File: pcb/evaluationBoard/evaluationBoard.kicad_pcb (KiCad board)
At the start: 2 copper layers, 36 parts, among them IC1 STM32F429ZGT6, IC2 TPS5430DDAR, IC3 TPS54331DR

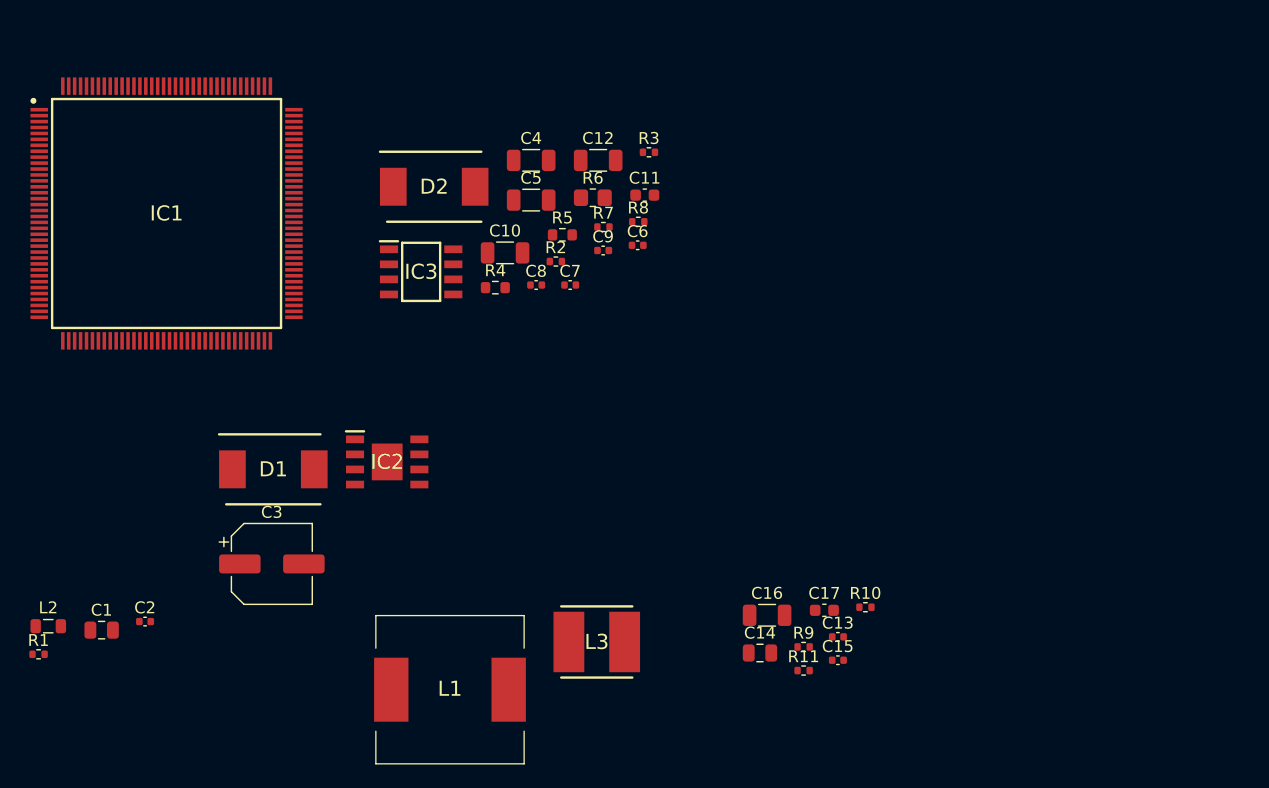
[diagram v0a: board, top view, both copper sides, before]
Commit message: wip
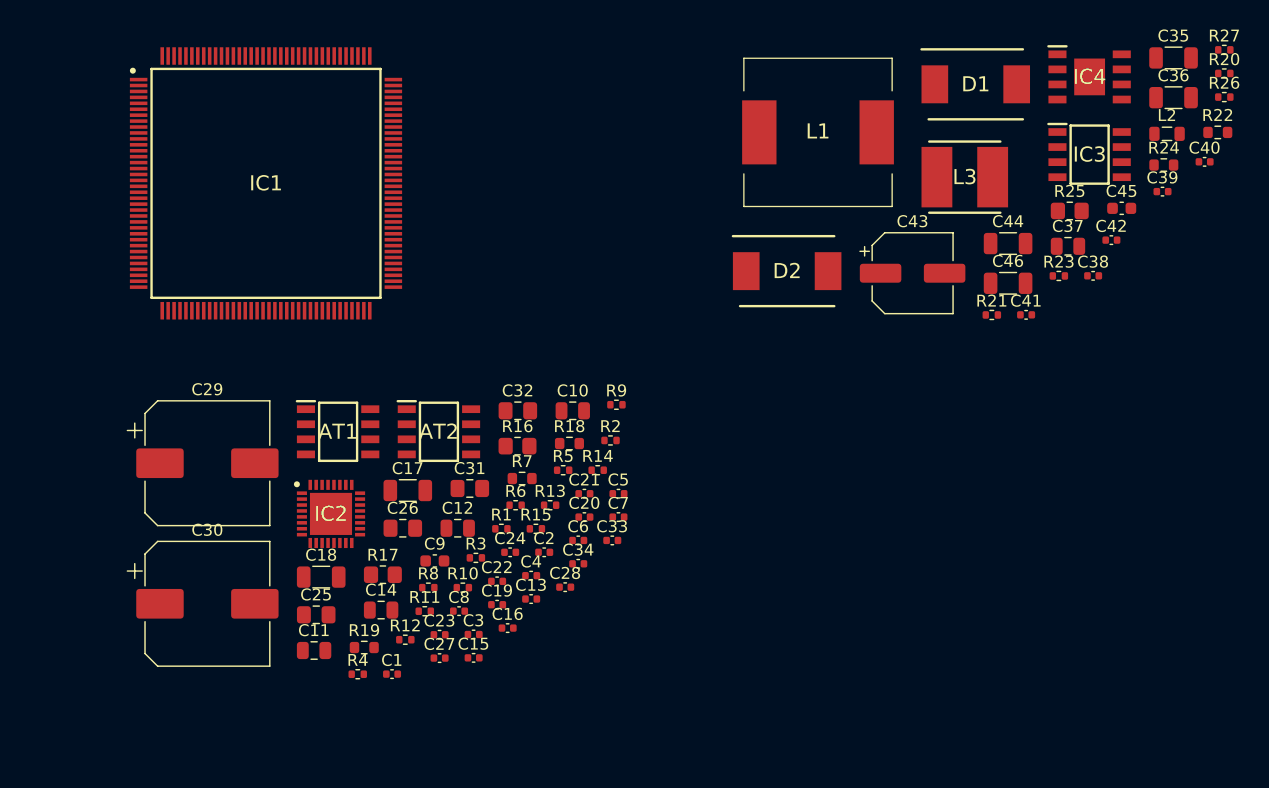
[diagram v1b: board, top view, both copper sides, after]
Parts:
- added AT1: LM386MX-1_NOPB, SOIC127P600X175-8N, F.Cu at (168.2, 72.8)
- added AT2: LM386MX-1_NOPB, SOIC127P600X175-8N, F.Cu at (176.7, 72.8)
- added C18: 47uF, Capacitor_SMD:C_1206_3216Metric, F.Cu at (166.8, 85.1)
- added C19: 4.7n, Capacitor_SMD:C_0402_1005Metric, F.Cu at (181.6, 87.4)
- added C20: 4.7n, Capacitor_SMD:C_0402_1005Metric, F.Cu at (189.0, 80.0)
- added C21: 100n, Capacitor_SMD:C_0402_1005Metric, F.Cu at (189.0, 78.0)
- added C22: 100n, Capacitor_SMD:C_0402_1005Metric, F.Cu at (181.6, 85.4)
- added C23: 100n, Capacitor_SMD:C_0402_1005Metric, F.Cu at (176.8, 89.9)
- added C24: 100n, Capacitor_SMD:C_0402_1005Metric, F.Cu at (182.7, 83.0)
- added C25: NA_C, Capacitor_SMD:C_0805_2012Metric_Pad1.18x1.45mm_HandSolder, F.Cu at (166.4, 88.3)
- added C26: NA_C, Capacitor_SMD:C_0805_2012Metric_Pad1.18x1.45mm_HandSolder, F.Cu at (173.7, 81.0)
- added C27: 47n, Capacitor_SMD:C_0402_1005Metric, F.Cu at (176.8, 91.9)
- added C28: 47n, Capacitor_SMD:C_0402_1005Metric, F.Cu at (187.3, 85.9)
- added C29: 220uF_E, Capacitor_SMD:CP_Elec_10x10, F.Cu at (157.2, 75.5)
- added C30: 220uF_E, Capacitor_SMD:CP_Elec_10x10, F.Cu at (157.2, 87.3)
- added C31: NA_C, Capacitor_SMD:C_0805_2012Metric_Pad1.18x1.45mm_HandSolder, F.Cu at (179.3, 77.6)
- added C32: NA_C, Capacitor_SMD:C_0805_2012Metric_Pad1.18x1.45mm_HandSolder, F.Cu at (183.4, 71.1)
- added C33: 100n, Capacitor_SMD:C_0402_1005Metric, F.Cu at (191.3, 82.0)
- added C34: 100n, Capacitor_SMD:C_0402_1005Metric, F.Cu at (188.4, 84.0)
- added C35: 4.7u, Capacitor_SMD:C_1206_3216Metric, F.Cu at (238.6, 41.3)
- added C36: 4.7u, Capacitor_SMD:C_1206_3216Metric, F.Cu at (238.6, 44.7)
- added C37: 10u, Capacitor_SMD:C_0805_2012Metric, F.Cu at (229.7, 57.2)
- added C38: 10n, Capacitor_SMD:C_0402_1005Metric, F.Cu at (231.9, 59.7)
- added C39: 100n, Capacitor_SMD:C_0402_1005Metric, F.Cu at (237.7, 52.6)
- added C40: 10n, Capacitor_SMD:C_0402_1005Metric, F.Cu at (241.3, 50.1)
- added C41: 10n, Capacitor_SMD:C_0402_1005Metric, F.Cu at (226.2, 63.0)
- added C42: 1n, Capacitor_SMD:C_0402_1005Metric, F.Cu at (233.4, 56.7)
- added C43: 220uF_E, Capacitor_SMD:CP_Elec_6.3x7.7, F.Cu at (216.6, 59.5)
- added C44: 47uF, Capacitor_SMD:C_1206_3216Metric, F.Cu at (224.7, 57.0)
- added C45: 47pF, Capacitor_SMD:C_0603_1608Metric, F.Cu at (234.3, 54.0)
- added C46: 47uF, Capacitor_SMD:C_1206_3216Metric, F.Cu at (224.7, 60.3)
- added IC4: TPS5430DDAR, SOIC127P600X170-9N, F.Cu at (231.6, 42.9)
- added R12: 1k, Resistor_SMD:R_0402_1005Metric, F.Cu at (173.9, 90.4)
- added R13: 2.7k, Resistor_SMD:R_0402_1005Metric, F.Cu at (186.1, 79.0)
- added R14: 1k, Resistor_SMD:R_0402_1005Metric, F.Cu at (190.1, 76.1)
- added R15: 1k, Resistor_SMD:R_0402_1005Metric, F.Cu at (184.9, 81.0)
- added R16: NA_R, Resistor_SMD:R_0805_2012Metric_Pad1.20x1.40mm_HandSolder, F.Cu at (183.3, 74.0)
- added R17: NA_R, Resistor_SMD:R_0805_2012Metric_Pad1.20x1.40mm_HandSolder, F.Cu at (172.0, 84.9)
- added R18: 10, Resistor_SMD:R_0603_1608Metric, F.Cu at (187.7, 73.8)
- added R19: 10, Resistor_SMD:R_0603_1608Metric, F.Cu at (170.4, 91.0)
- added R20: 330k, Resistor_SMD:R_0402_1005Metric, F.Cu at (242.9, 42.6)
- added R21: 68k, Resistor_SMD:R_0402_1005Metric, F.Cu at (223.3, 63.0)
- added R22: 30k, Resistor_SMD:R_0603_1608Metric, F.Cu at (242.4, 47.6)
- added R23: 10k, Resistor_SMD:R_0402_1005Metric, F.Cu at (229.0, 59.7)
- added R24: 3k, Resistor_SMD:R_0603_1608Metric, F.Cu at (237.8, 50.3)
- added R25: 0, Resistor_SMD:R_0805_2012Metric_Pad1.20x1.40mm_HandSolder, F.Cu at (229.9, 54.2)
- added R26: 10k, Resistor_SMD:R_0402_1005Metric, F.Cu at (242.9, 44.6)
- added R27: 3.3k, Resistor_SMD:R_0402_1005Metric, F.Cu at (242.9, 40.6)
- C1: value 10u -> 33p; footprint Capacitor_SMD:C_0805_2012Metric -> Capacitor_SMD:C_0402_1005Metric
- C10, C12: value 47uF -> 10u; footprint Capacitor_SMD:C_1206_3216Metric -> Capacitor_SMD:C_0805_2012Metric
- C11: value 47pF -> 10u; footprint Capacitor_SMD:C_0603_1608Metric -> Capacitor_SMD:C_0805_2012Metric
- C15: value 47n -> 100n
- C16: value 47uF -> 100n; footprint Capacitor_SMD:C_1206_3216Metric -> Capacitor_SMD:C_0402_1005Metric
- C17: value 1u -> 47uF; footprint Capacitor_SMD:C_0603_1608Metric -> Capacitor_SMD:C_1206_3216Metric
- C2: value 10n -> 100n
- C3: value 220uF_E -> 100n; footprint Capacitor_SMD:CP_Elec_6.3x7.7 -> Capacitor_SMD:C_0402_1005Metric
- C4, C5: value 4.7u -> 100n; footprint Capacitor_SMD:C_1206_3216Metric -> Capacitor_SMD:C_0402_1005Metric
- C6, C8: value 10n -> 33p
- C7: value 100n -> 33p
- C9: value 1n -> 1u; footprint Capacitor_SMD:C_0402_1005Metric -> Capacitor_SMD:C_0603_1608Metric
- IC2: value TPS5430DDAR -> TLV320AIC3254IRHBT; footprint SOIC127P600X170-9N -> SamacSys_Parts:QFN50P500X500X100-33N-D
- R1: value 10k -> 22
- R10, R9: value 1k -> 22
- R11: value 2.7k -> 1k
- R2: value 330k -> 22
- R3: value 68k -> 22
- R4: value 30k -> 22; footprint Resistor_SMD:R_0603_1608Metric -> Resistor_SMD:R_0402_1005Metric
- R5: value 3k -> 1k; footprint Resistor_SMD:R_0603_1608Metric -> Resistor_SMD:R_0402_1005Metric
- R6: value 0 -> 1k; footprint Resistor_SMD:R_0805_2012Metric_Pad1.20x1.40mm_HandSolder -> Resistor_SMD:R_0402_1005Metric
- R7: value 10k -> 10; footprint Resistor_SMD:R_0402_1005Metric -> Resistor_SMD:R_0603_1608Metric
- R8: value 3.3k -> 22
- moved L2 103.1 mm to (238.1, 47.7)
- moved D1 67.5 mm to (222.0, 43.5)
- moved IC3 57.2 mm to (231.6, 49.5)
- moved L1 56.3 mm to (208.7, 47.6)
- moved L3 50.0 mm to (221.0, 51.4)
- moved C11 47.5 mm to (166.2, 91.3)
- moved R1 40.4 mm to (182.0, 81.0)
- moved R3 37.2 mm to (179.8, 83.5)
- moved C17 36.5 mm to (174.1, 77.8)
- moved R8 35.6 mm to (175.8, 86.0)
- moved C4 35.0 mm to (184.5, 85.0)
- moved R4 34.6 mm to (169.9, 93.3)
- moved C2 34.2 mm to (185.6, 83.0)
- moved R10 34.0 mm to (178.7, 86.0)
- moved C12 33.2 mm to (178.3, 81.0)
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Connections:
- net Net-(C15-Pad1) renamed /dsp/MIC-
- net Net-(C17-Pad1) renamed /dsp/-HPL
- net Net-(R10-Pad2) renamed /dsp/SDA
- net Net-(R9-Pad2) renamed /dsp/DOUT
- C1 pad 1: +VDC -> Net-(C1-Pad1)
- C10 pad 1: +3V3 -> Net-(C10-Pad1)
- C11 pad 1: Net-(C11-Pad1) -> +3V3
- C12 pad 1: +3V3 -> Net-(C10-Pad1)
- C13 pad 1: Net-(C13-Pad1) -> +3V3
- C13 pad 2: Net-(C13-Pad2) -> GND
- C14 pad 1: Net-(C14-Pad1) -> Net-(C10-Pad1)
- C14 pad 2: Net-(C14-Pad2) -> GND
- C16 pad 1: Net-(C16-Pad1) -> /dsp/MIC+
- C2 pad 1: Net-(C2-Pad1) -> Net-(C1-Pad1)
- C2 pad 2: Net-(C2-Pad2) -> /dsp/-IN1_L
- C3 pad 1: +5V -> Net-(C3-Pad1)
- C3 pad 2: GND -> /dsp/-IN1_R
- C4 pad 1: +VDC -> Net-(C4-Pad1)
- C4 pad 2: GND -> /dsp/-IN2_L
- C5 pad 1: +VDC -> Net-(C5-Pad1)
- C5 pad 2: GND -> /dsp/-IN2_R
- C6 pad 1: +VDC -> Net-(C3-Pad1)
- C7 pad 1: Net-(C7-Pad1) -> Net-(C4-Pad1)
- C7 pad 2: Net-(C7-Pad2) -> GND
- C8 pad 1: Net-(C8-Pad1) -> Net-(C5-Pad1)
- C9 pad 1: Net-(C11-Pad1) -> +3V3
- C9 pad 2: Net-(C9-Pad2) -> GND
- D1 pad 1: Net-(C2-Pad1) -> Net-(C41-Pad1)
- D2 pad 1: Net-(C7-Pad1) -> Net-(C39-Pad1)
- IC2 pad 1: Net-(C2-Pad2) -> Net-(IC2-Pad1)
- IC2 pad 5: /power/ENA -> Net-(IC2-Pad5)
- IC2 pad 6: GND -> +3V3
- IC2 pad 7: +VDC -> GND
- IC2 pad 8: Net-(C2-Pad1) -> /dsp/MIC+
- IC2 pad 9: GND -> Net-(IC2-Pad9)
- IC3 pad 1: Net-(C7-Pad2) -> Net-(C39-Pad2)
- IC3 pad 4: Net-(C8-Pad1) -> Net-(C40-Pad1)
- IC3 pad 6: Net-(C11-Pad1) -> Net-(C42-Pad1)
- IC3 pad 8: Net-(C7-Pad1) -> Net-(C39-Pad1)
- L1 pad 1: Net-(C2-Pad1) -> Net-(C41-Pad1)
- L3 pad 1: Net-(C7-Pad1) -> Net-(C39-Pad1)
- R1 pad 1: +5V -> Net-(IC2-Pad2)
- R1 pad 2: Net-(IC2-Pad4) -> /dsp/BCLK
- R10 pad 1: Net-(R10-Pad1) -> Net-(IC2-Pad10)
- R11 pad 1: Net-(R11-Pad1) -> MICBIAS
- R11 pad 2: Net-(R11-Pad2) -> /dsp/-IN1_L
- R2 pad 1: +VDC -> Net-(IC2-Pad4)
- R2 pad 2: Net-(IC3-Pad3) -> /dsp/DIN
- R3 pad 1: Net-(IC3-Pad3) -> Net-(IC2-Pad9)
- R3 pad 2: GND -> /dsp/SCL
- R4 pad 1: Net-(C9-Pad2) -> Net-(IC2-Pad11)
- R4 pad 2: GND -> /dsp/MISO
- R5 pad 1: Net-(IC2-Pad4) -> MICBIAS
- R5 pad 2: GND -> /dsp/-IN2_L
- R6 pad 1: +3V3 -> /dsp/-IN2_R
- R6 pad 2: Net-(R6-Pad2) -> GND
- R7 pad 1: Net-(R6-Pad2) -> Net-(IC2-Pad1)
- R7 pad 2: Net-(IC3-Pad5) -> /dsp/MCLK
- R8 pad 1: Net-(IC3-Pad5) -> Net-(IC2-Pad3)
- R8 pad 2: GND -> /dsp/WCLK
- R9 pad 1: Net-(R9-Pad1) -> Net-(IC2-Pad5)
